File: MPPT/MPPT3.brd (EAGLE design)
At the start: 92 parts, among them X1 22-23-2021, X2 22-23-2021, X3 22-23-2041

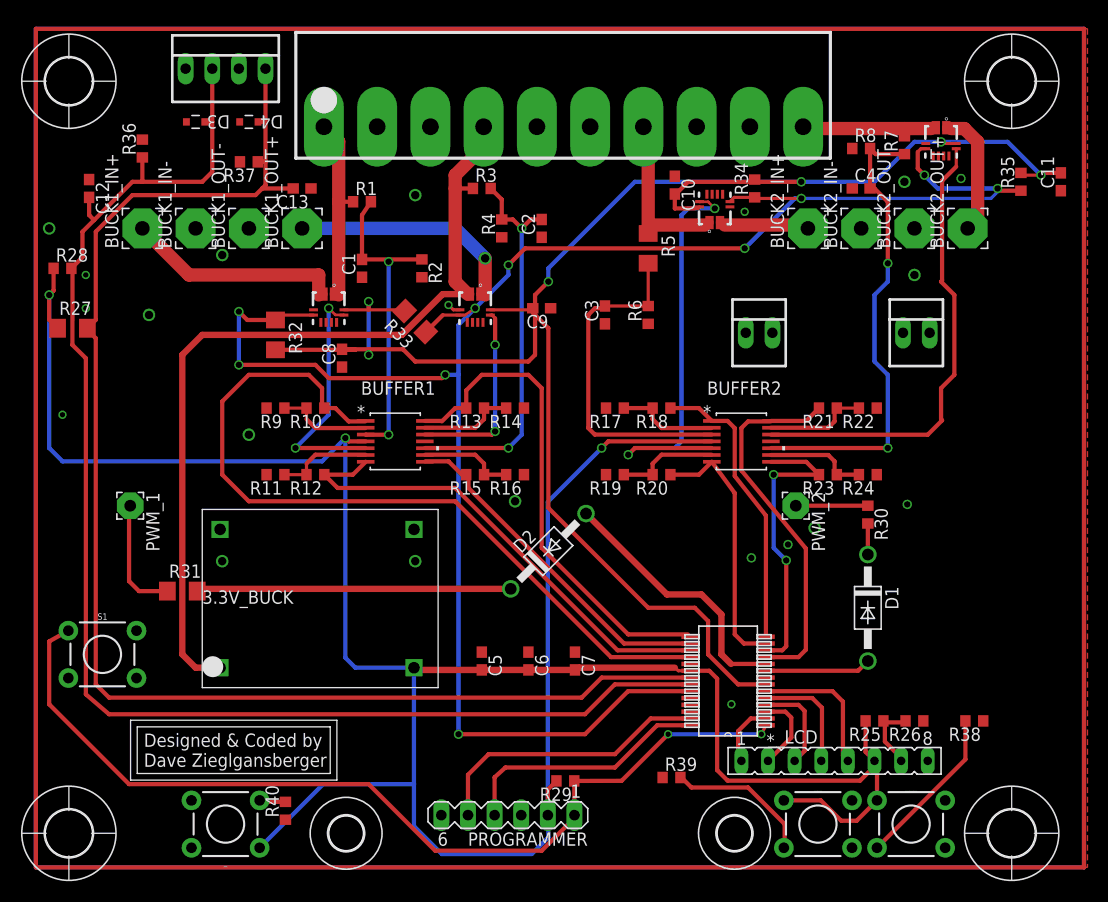
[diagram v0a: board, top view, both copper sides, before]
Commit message: SendOutForFab
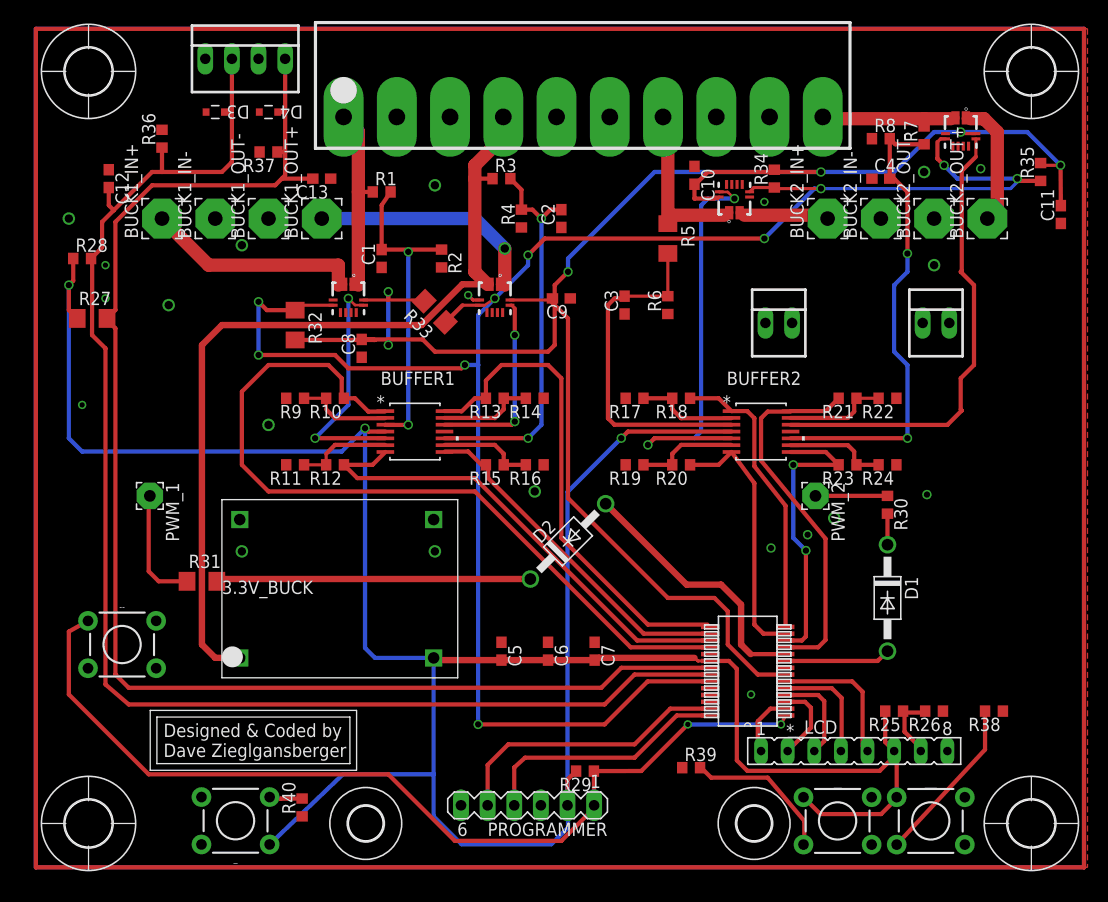
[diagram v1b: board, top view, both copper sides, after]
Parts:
- removed S1: Reset, SparkFun-Switches:TACTILE_SWITCH_PTH_6.0MM
- added --: Reset, SparkFun-Switches:TACTILE_SWITCH_PTH_6.0MM
- moved C11 3.12 mm to (97.8, 62.3)
- moved C1 2.10 mm to (33.0, 58.1)
- moved R1 2.10 mm to (33.0, 64.4)
- moved U$2 2.10 mm to (5.03, 75.9)
- moved U$4 2.10 mm to (5.03, 4.19)
- moved 3.3V_BUCK 2.10 mm to (17.8, 18.1)
- moved B1_I 2.10 mm to (43.8, 54.3)
- moved B2_I 2.10 mm to (88.2, 70.2)
- moved BUCK1_IN+ 2.10 mm to (12.0, 61.9)
- moved BUCK1_OUT+ 2.10 mm to (27.3, 61.9)
- moved BUCK1_OUT- 2.10 mm to (22.2, 61.9)
- moved BUCK2_IN+ 2.10 mm to (75.5, 61.9)
- moved BUCK2_IN- 2.10 mm to (80.6, 61.9)
- moved BUCK2_OUT+ 2.10 mm to (90.8, 61.9)
- moved BUCK2_OUT- 2.10 mm to (85.7, 61.9)
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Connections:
- net N$40: now also --.1; no longer S1.1
- net VSS: now also --.3; no longer S1.3
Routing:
- net N$53: track 178.4 -> 180.5 mm
- net VDD: track 254.6 -> 256.1 mm
- net N$51: track 2.52 -> 3.11 mm
